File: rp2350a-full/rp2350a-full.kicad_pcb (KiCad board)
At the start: 2 copper layers, 20.3 x 48.3 mm, 43 parts, among them J1 USB2.0-C_SMT, J2 SWD_10Pin_MCU-Side, SW1 SKRPABE010, SW2 SKRPABE010, U1 RP2350A, U2 AMS1117, U3 W25Q32JVSS, U4 CH213K, Y1 12M

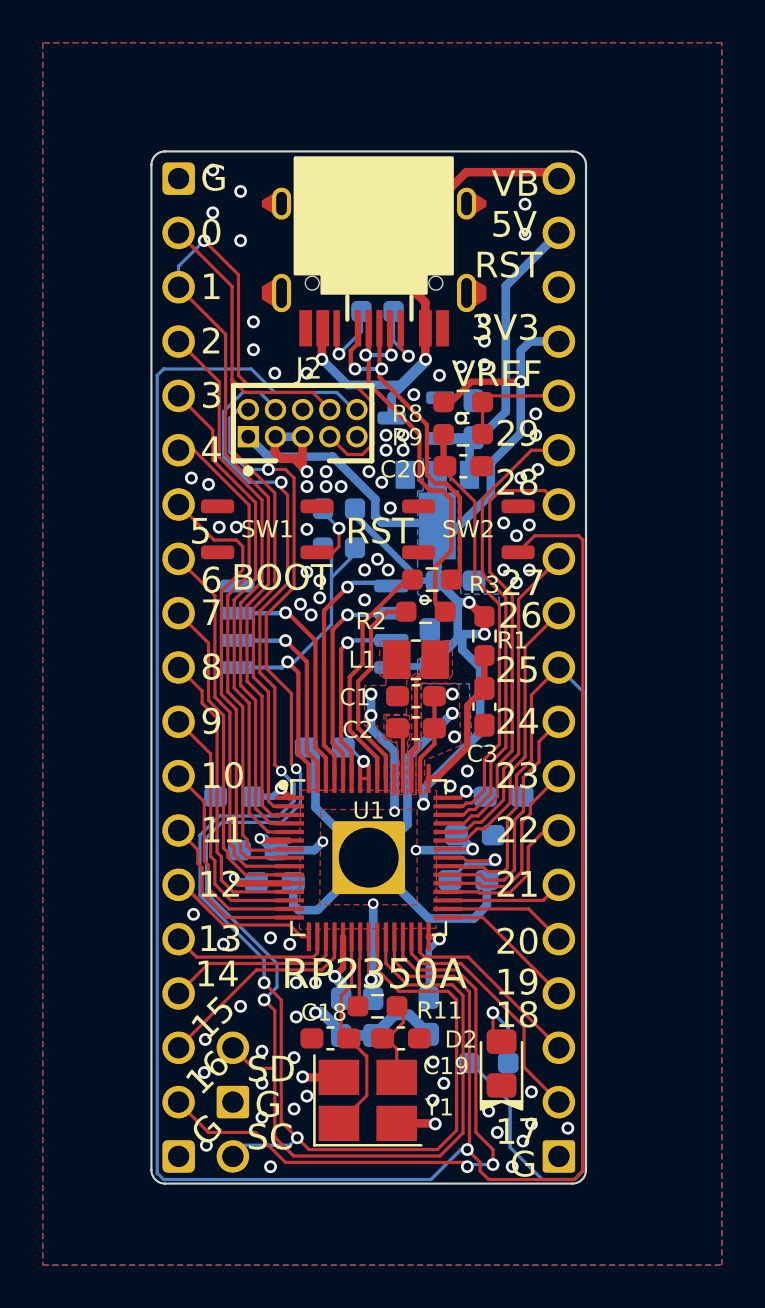
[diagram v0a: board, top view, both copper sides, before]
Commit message: fix
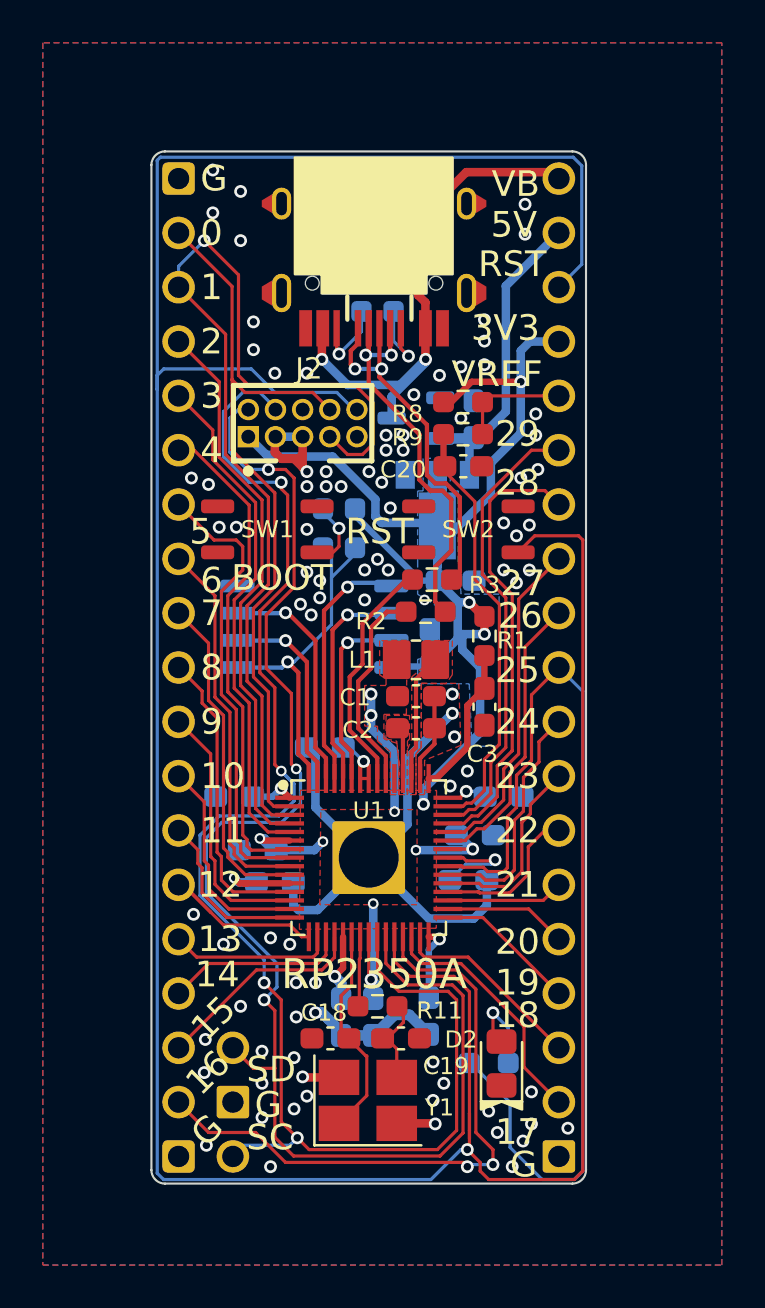
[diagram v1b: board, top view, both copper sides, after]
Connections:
- CH1 pad 36: /RESET -> /RUN
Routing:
- net /RUN: track 115.8 -> 152.7 mm
